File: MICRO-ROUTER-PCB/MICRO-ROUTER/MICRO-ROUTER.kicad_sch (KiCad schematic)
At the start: 72 parts, among them J2 USB_A, J3 USB_C_Receptacle_USB2.0_16P, J4 Battery Connector, J5 SPI Header, J6 GPIO Header, J7 RJ45 5-2301996-6, Q1 FS8205A, SW2 8Devices Reset, SW3 UART Reset, U1 TP4056, U2 XC9142B33DMR-G, U3 CP2102N-Axx-xQFN20, U4 DW01A, X1 142-0711-821

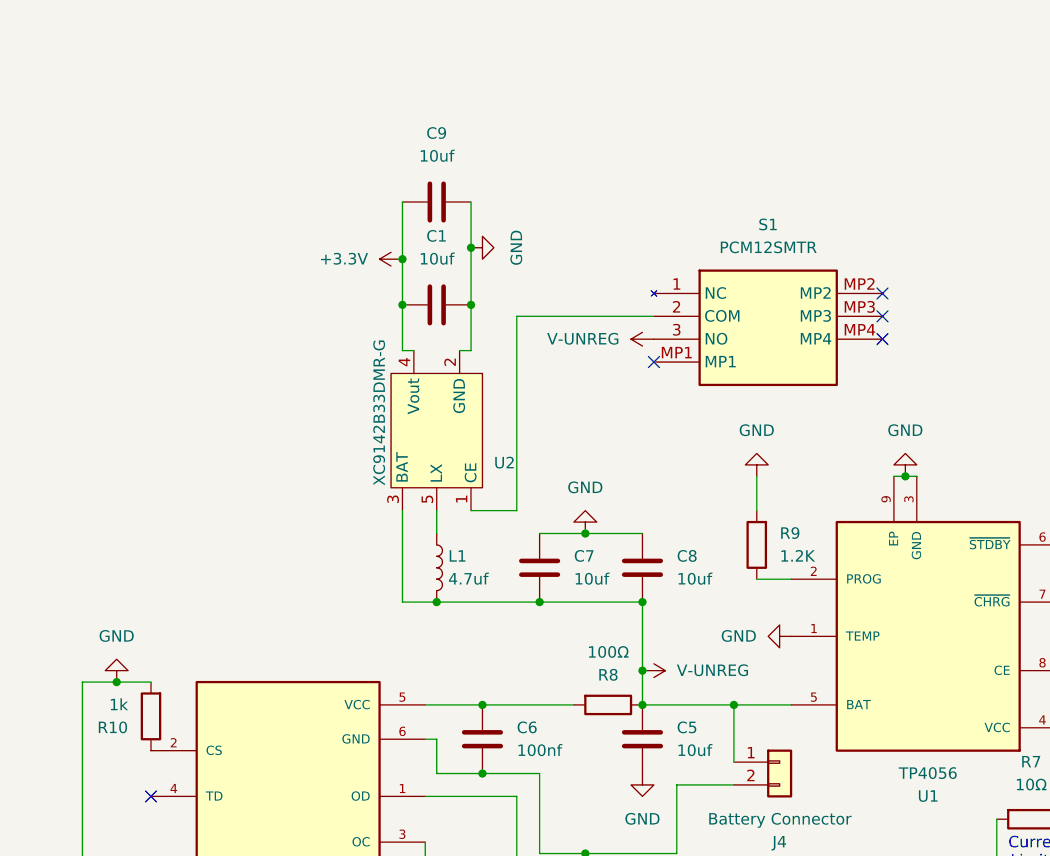
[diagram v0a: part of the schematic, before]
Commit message: fixed reg
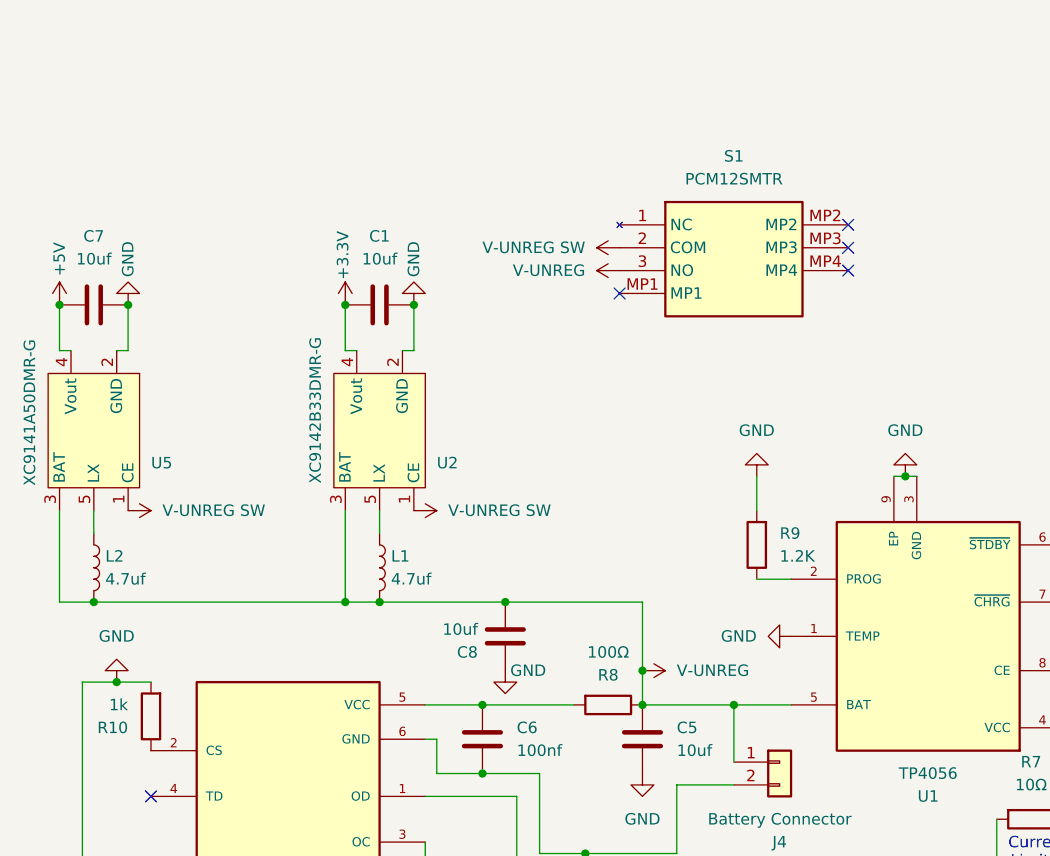
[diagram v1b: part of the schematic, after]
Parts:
- removed C9: 10uf, Capacitor_SMD:C_0603_1608Metric, symbol Device:C
- added L2: 4.7uf, Custom Footprints:INDPM5752X300N, symbol Device:L
- added U5: XC9141A50DMR-G, Custom Footprints:XC8107AC20MR-G, symbol Custom Symbols:XC9142B33DMR-G
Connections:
- net +5V: now also C7.1, U5.4 (Vout)
- net GND: now also U5.2 (GND)
- net V-UNREG: now also L2.2, U5.3 (BAT); no longer C7.1
- net V-UNREG SW: now reaches S1.2 (COM), U2.1 (CE)
- net V-UNREG SW: now also U5.1 (CE)
- new net: L2.1, U5.5 (LX)
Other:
- moved on the sheet: C1, C8, L1, S1, U2
